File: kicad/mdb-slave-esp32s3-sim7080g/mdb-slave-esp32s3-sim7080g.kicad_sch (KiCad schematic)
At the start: 81 parts, among them J1 USB_C_Receptacle_USB2.0_16P, J2 JAE_SIM_Card_SF72S006, J3 Conn_01x03_Pin, J4 Conn_Coaxial, J5 Conn_Coaxial, J6 MDB_Connector, J7 Conn_01x03_Pin, J8 Conn_01x04_Pin, Q1 MMBT3904, Q2 MMBT3904, Q3 MMBT3904, Q4 MMBT3904, Q5 MMBT3904, Q6 MMBT3904, Q7 MMBT3904, SW1 SW_Push, U1 ESP32-S3FH4R2, U2 SIM7080G, U3 LM2594HVM-3.3, U4 TLP785, U5 TLP785, Y1 Crystal_GND24

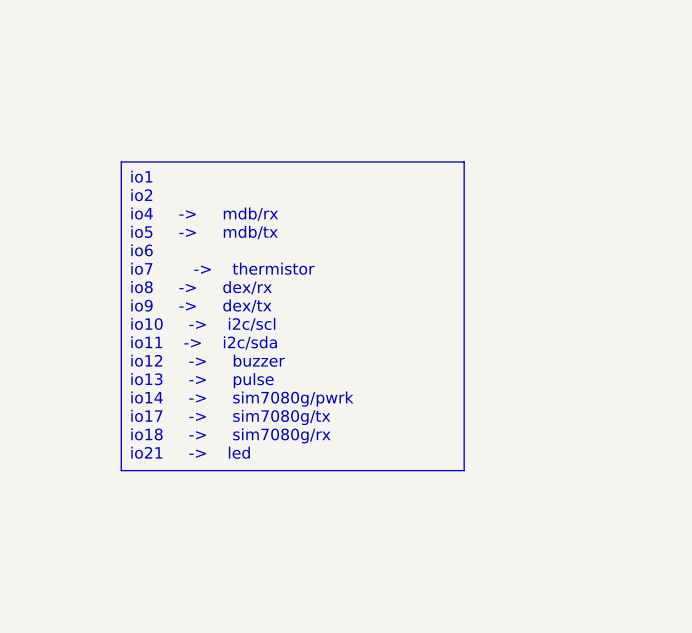
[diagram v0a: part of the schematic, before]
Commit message: routing...
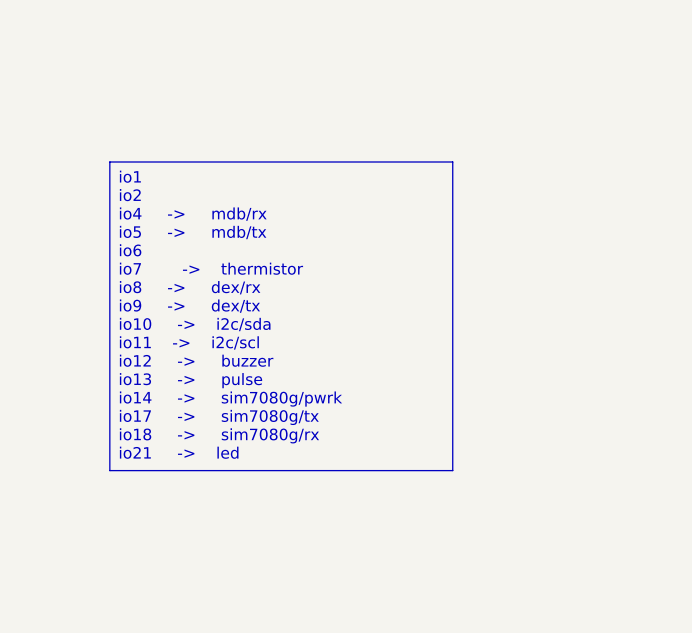
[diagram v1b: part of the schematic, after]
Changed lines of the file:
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@@
 		)
 	)
-	(text_box "io1\nio2\nio4 	-> 	mdb/rx\nio5 	-> 	mdb/tx\nio6 	\nio7		->	thermistor\nio8 	-> 	dex/rx\nio9 	-> 	dex/tx\nio10 	->	i2c/scl\nio11	->	i2c/sda\nio12 	-> 	buzzer\nio13 	-> 	pulse\nio14 	-> 	sim7080g/pwrk\nio17 	-> 	sim7080g/tx\nio18 	-> 	sim7080g/rx\nio21 	->	led	\n"
+	(text_box "MCU <-> sim7080G"
 		(exclude_from_sim no)
-		(at 31.75 168.91 0)
-		(size 38.1 34.29)
+		(at 52.07 294.64 0)
+		(size 63.5 82.55)
 		(margins 0.9525 0.9525 0.9525 0.9525)
 		(stroke
@@
 		)
 	)
-	(text_box "MCU <-> sim7080G"
+	(text_box "io1\nio2\nio4 	-> 	mdb/rx\nio5 	-> 	mdb/tx\nio6 	\nio7		->	thermistor\nio8 	-> 	dex/rx\nio9 	-> 	dex/tx\nio10 	->	i2c/sda\nio11	->	i2c/scl\nio12 	-> 	buzzer\nio13 	-> 	pulse\nio14 	-> 	sim7080g/pwrk\nio17 	-> 	sim7080g/tx\nio18 	-> 	sim7080g/rx\nio21 	->	led	\n"
 		(exclude_from_sim no)
-		(at 52.07 294.64 0)
-		(size 63.5 82.55)
+		(at 30.48 168.91 0)
+		(size 38.1 34.29)
 		(margins 0.9525 0.9525 0.9525 0.9525)
 		(stroke
